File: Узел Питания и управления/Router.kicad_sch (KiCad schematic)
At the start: 8 parts

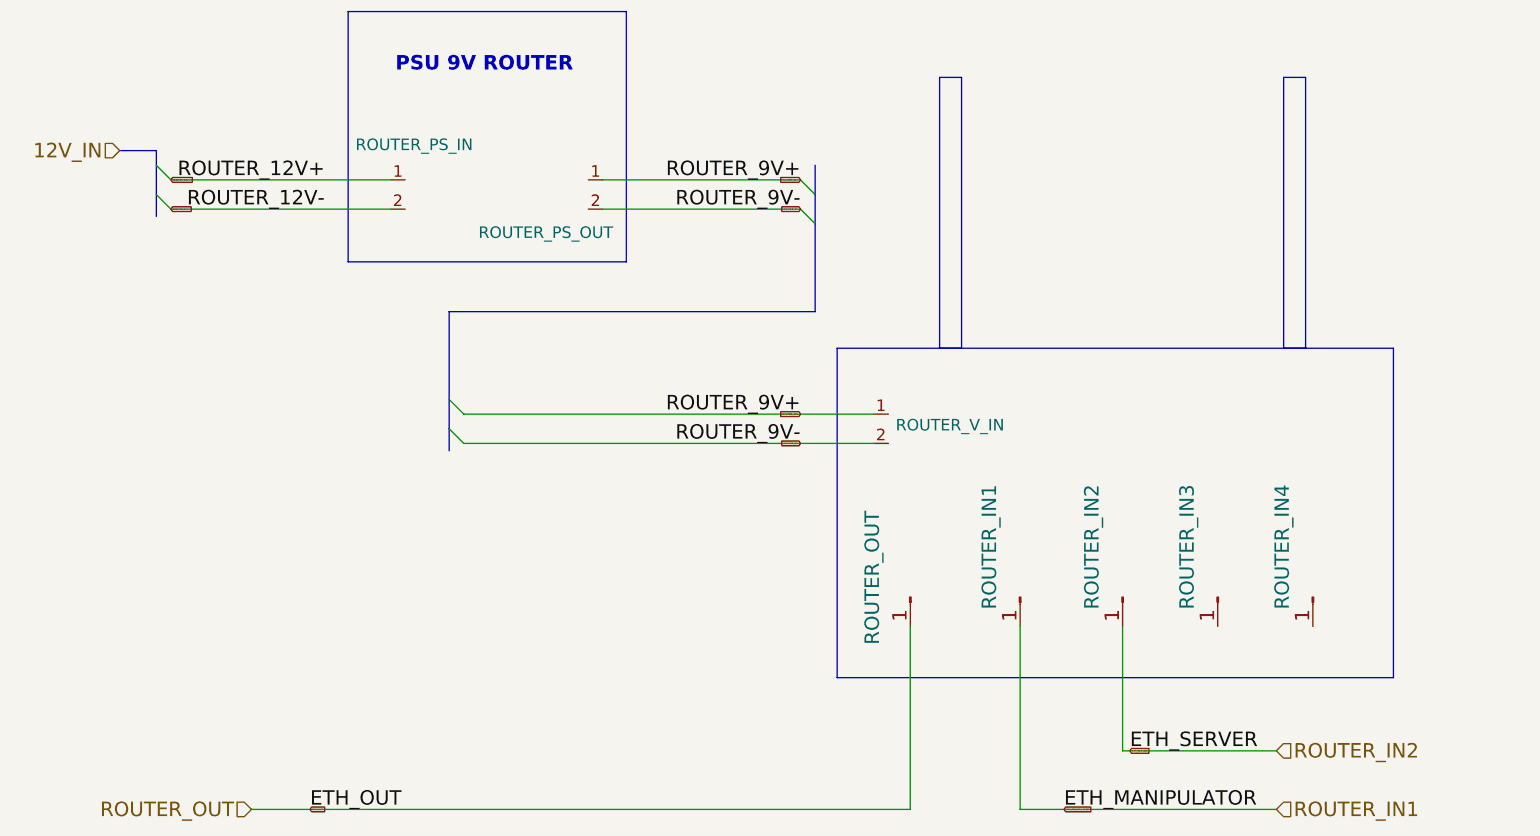
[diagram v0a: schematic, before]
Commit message: update schemas
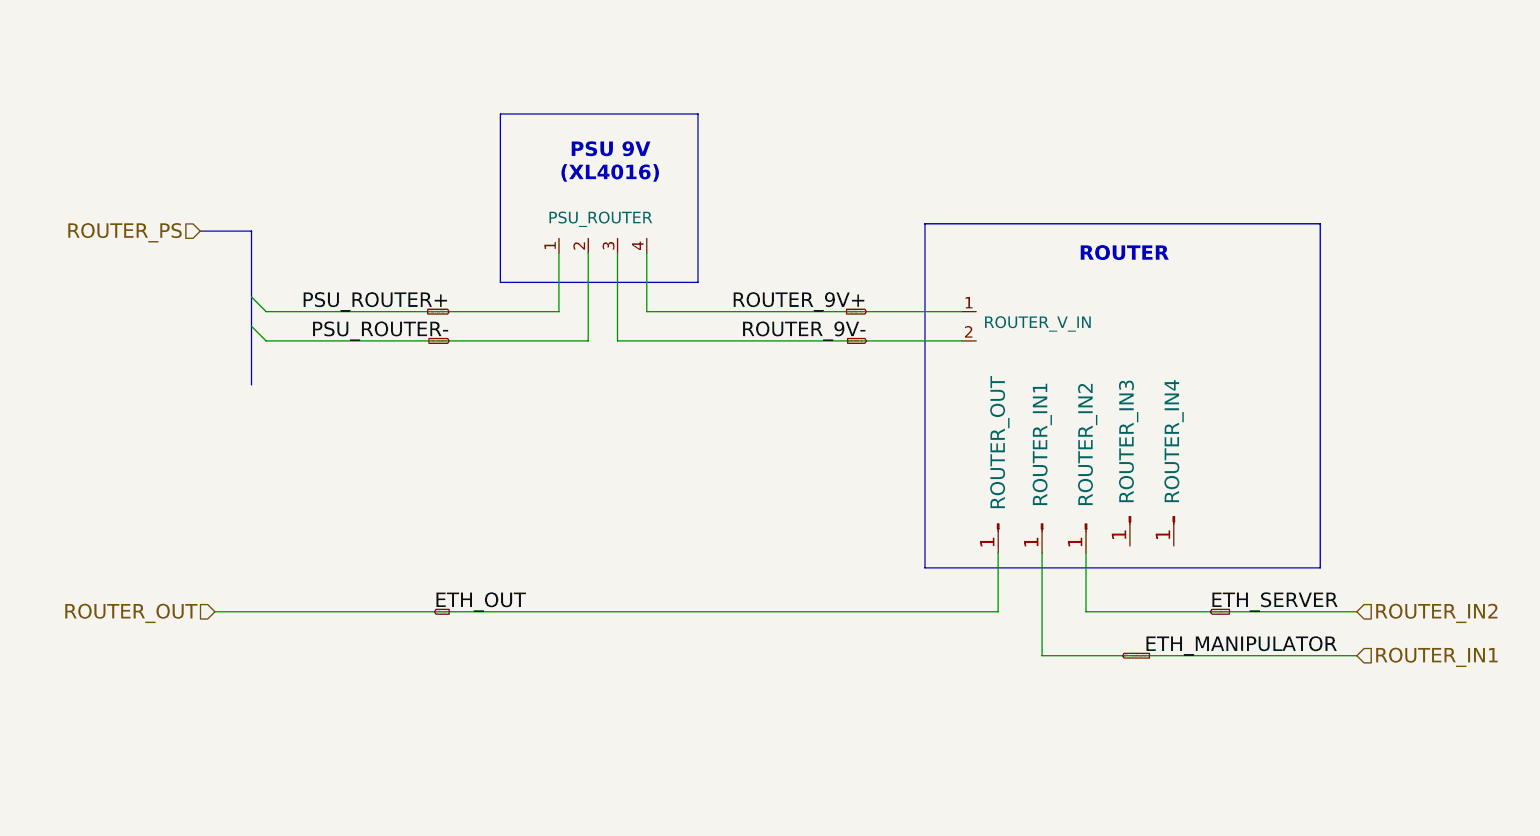
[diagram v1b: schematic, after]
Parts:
- removed ROUTER_PS_IN, ROUTER_PS_OUT: ~, symbol Connector:Conn_01x02_(wide)
- added PSU_ROUTER: ~, symbol Connector:Conn_01x04_(wide)
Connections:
- net ROUTER_9V+: now also PSU_ROUTER.4
- net ROUTER_9V-: now also PSU_ROUTER.3
- new net PSU_ROUTER+: PSU_ROUTER.1
- new net PSU_ROUTER-: PSU_ROUTER.2
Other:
- note added: "PSU 9V (XL4016)"
- note added: "ROUTER"
- note removed: "PSU 9V ROUTER"
- moved on the sheet: ROUTER_IN1, ROUTER_IN2, ROUTER_IN3, ROUTER_IN4, ROUTER_OUT, ROUTER_V_IN
